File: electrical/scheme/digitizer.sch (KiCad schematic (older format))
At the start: 173 parts, among them P1 mode, P10 in-2, P11 in-3, P12 in-1, P13 USB_B, P14 screw, P15 screw, P16 screw, P17 screw, P2 ~rst~, P3 ext, P4 trig, P5 trig-mode, P6 swd, P7 out-0, P8 out-1, P9 in-0, U1 AD8672, U10 crystal-4pin, U100 AD8672, U101 AD8672, U11 CP2102, U12 adr4533, U13 BAT54S, U14 adr4533, U15 ADT7410, U16 MCP1703T-3302E/CB, U17 AD7683, U18 NCP3063, U19 ADG5204, U2 AD8672, U20 NCP3063, U3 AD8672

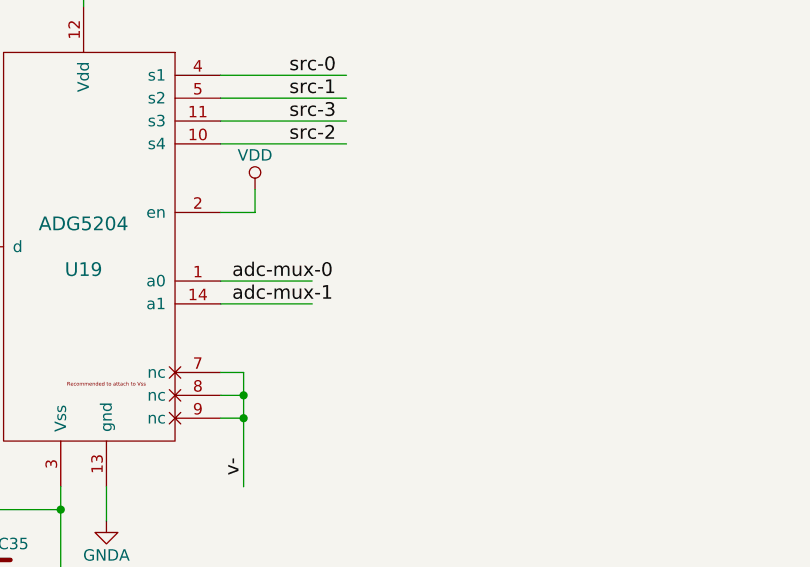
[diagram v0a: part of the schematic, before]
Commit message: a
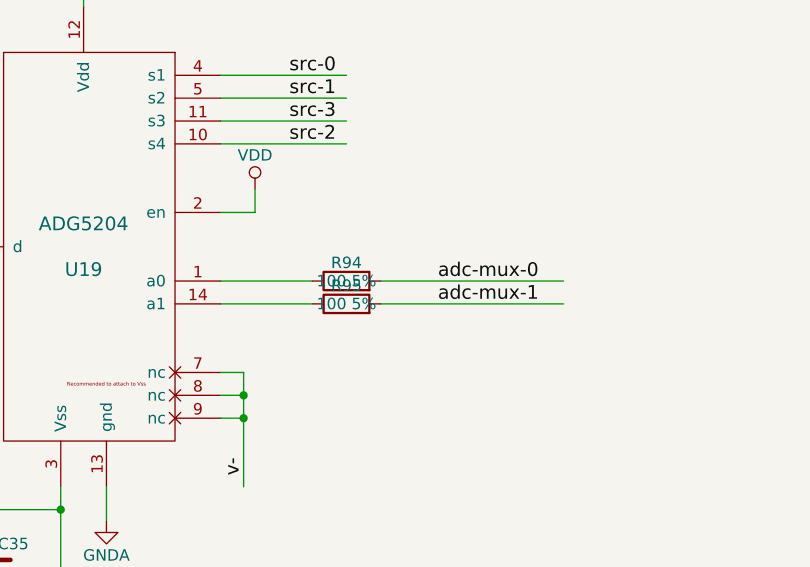
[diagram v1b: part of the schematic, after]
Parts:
- added R94, R95: 100 5%, Resistors_SMD:R_0805_HandSoldering, symbol R
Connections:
- wire segments 571 -> 573
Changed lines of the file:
@@
 	1    0    0    -1
 $EndComp
-Text Label 22950 2550 0    60   ~ 0
+Text Label 23850 2550 0    60   ~ 0
 adc-mux-0
-Text Label 22950 2650 0    60   ~ 0
+Text Label 23850 2650 0    60   ~ 0
 adc-mux-1
 $Comp
@@
 	1    0    0    -1
 $EndComp
+$Comp
+L R R94
+U 1 1 55A94CE2
+P 23450 2550
+F 0 "R94" V 23530 2550 50  0000 C CNN
+F 1 "100 5%" V 23450 2550 50  0000 C CNN
+F 2 "Resistors_SMD:R_0805_HandSoldering" V 23380 2550 30  0001 C CNN
+F 3 "" H 23450 2550 30  0000 C CNN
+	1    23450 2550
+	0    -1   -1   0
+$EndComp
+$Comp
+L R R95
+U 1 1 55A9753A
+P 23450 2650
+F 0 "R95" V 23530 2650 50  0000 C CNN
+F 1 "100 5%" V 23450 2650 50  0000 C CNN
+F 2 "Resistors_SMD:R_0805_HandSoldering" V 23380 2650 30  0001 C CNN
+F 3 "" H 23450 2650 30  0000 C CNN
+	1    23450 2650
+	0    -1   -1   0
+$EndComp
+Wire Wire Line
+	23600 2550 24400 2550
+Wire Wire Line
+	23600 2650 24400 2650
 $EndSCHEMATC
